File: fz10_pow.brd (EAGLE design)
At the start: 107 x 100 mm, 85 parts

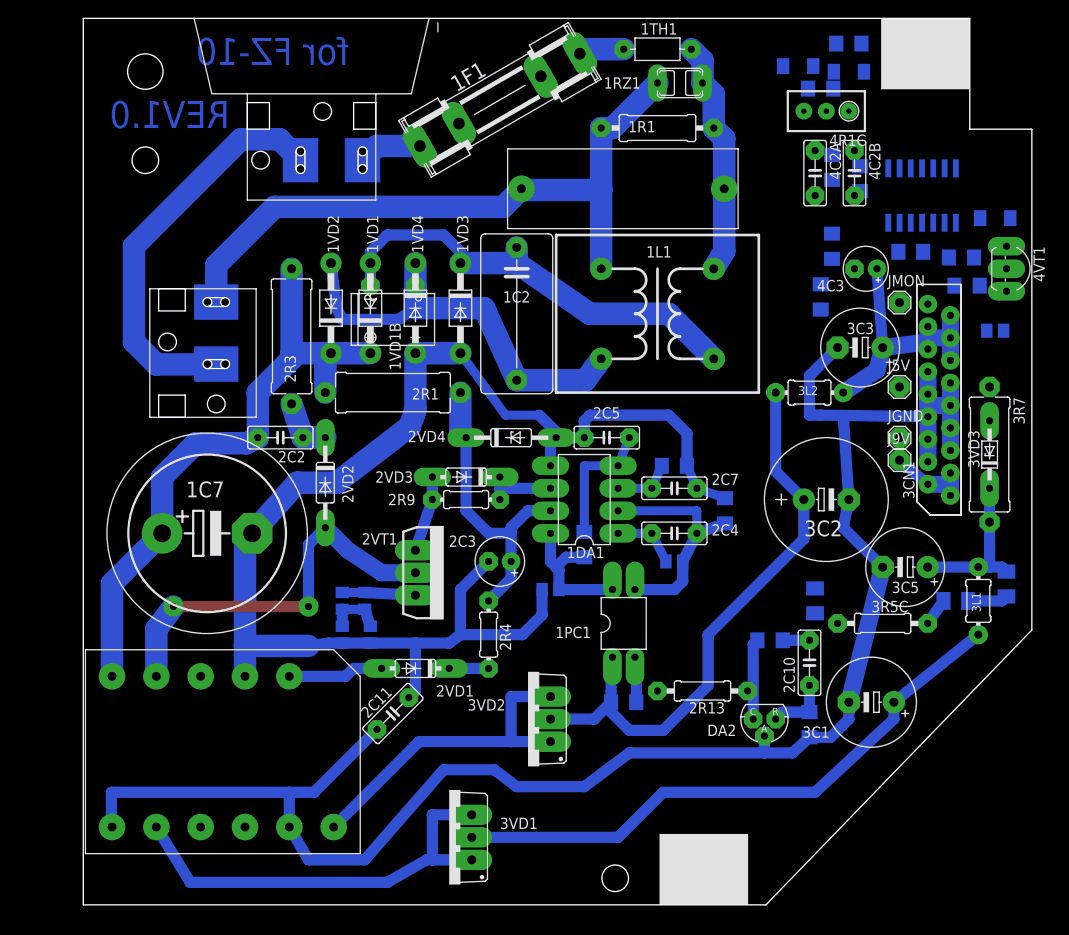
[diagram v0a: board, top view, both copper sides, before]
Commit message: .
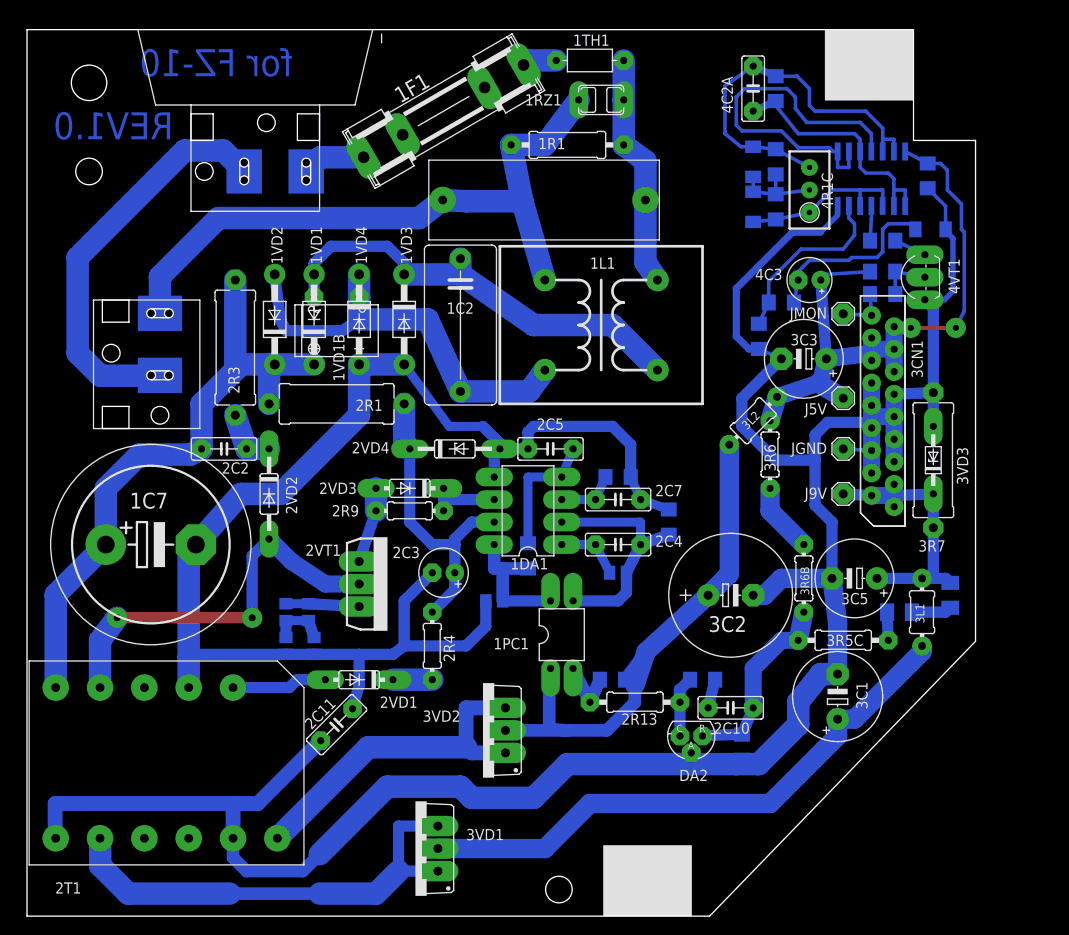
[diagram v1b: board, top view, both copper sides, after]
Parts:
- removed 4C2B: (no value), rcl:C050-025X075
- removed 4C2D: (no value), rcl:C1206
- added 3R6B: 0, rcl:0204/7
- 3R6: device rcl:M1206 -> rcl:0204/7
- 4R6: device rcl:M0805 -> rcl:R1206
- moved 4R1B 20.2 mm to (84.5, 80.0), turned to 270 degrees
- moved 4VD2 18.7 mm to (81.9, 80.0), turned to 270 degrees
- moved 3R6 17.3 mm to (83.8, 52.1), flipped to the top
- moved 3C2 15.3 mm to (79.4, 36.2)
- moved 4C2C 13.9 mm to (84.5, 93.3), turned to 90 degrees
- moved 4R6 13.4 mm to (96.5, 70.2)
- moved 4VD1 11.9 mm to (81.9, 85.1), turned to 90 degrees
- moved 4C2A 11.8 mm to (81.9, 93.3), turned to 90 degrees
- moved 4R4 10.8 mm to (96.5, 76.2)
- moved 1R1 10.3 mm to (61.0, 87.0)
- moved 2C10 10.2 mm to (79.4, 23.5), turned to 180 degrees
- moved 4R1A 9.69 mm to (84.5, 85.1), turned to 270 degrees
- moved 4VT1 9.26 mm to (101.3, 72.1), turned to 90 degrees
- moved 1RZ1 9.09 mm to (64.8, 92.1)
- moved 4R1C 9.09 mm to (88.3, 81.9), turned to 0 degrees
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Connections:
- new net N$43: 3R6.1, 3R6B.2
- net N$1: now also 4DD1.12, 4DD1.13; no longer 4C2B.2, 4C2D.2, 4DD1.1, 4DD1.2
- net N$19: now also 4DD1.1, 4DD1.10, 4DD1.2; no longer 4C2B.1, 4C2D.1, 4DD1.12, 4DD1.13, 4DD1.4
- net N$2: now also 4DD1.11, 4DD1.8, 4DD1.9; no longer 4DD1.3, 4DD1.5, 4DD1.6
- net N$25: now also 4DD1.4; no longer 4DD1.10
- net N$31: now also 4DD1.6; no longer 4DD1.8
- net N$42: now also 3R6B.1; no longer 3R6.1
- net N$7: now also 4DD1.3, 4DD1.5; no longer 4DD1.11, 4DD1.9
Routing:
- net GND: track 196.5 -> 277.0 mm
- net +5V: track 31.4 -> 75.2 mm, vias 0 -> 2
- net N$1: track 0.00 -> 43.5 mm
- net N$2: track 0.00 -> 41.4 mm
- net N$19: track 0.00 -> 28.3 mm
- net N$35: track 0.00 -> 20.7 mm
- net N$31: track 0.00 -> 20.5 mm
- net N$7: track 0.00 -> 19.4 mm
- net N$42: track 7.16 -> 21.8 mm
- net N$10: track 0.00 -> 10.3 mm
- net N$43: track 0.00 -> 7.93 mm
- net N$29: track 0.00 -> 5.94 mm
- net MON: track 0.00 -> 5.61 mm
- net N$13: track 66.4 -> 62.3 mm
- net N$25: track 0.00 -> 3.92 mm
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
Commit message: .
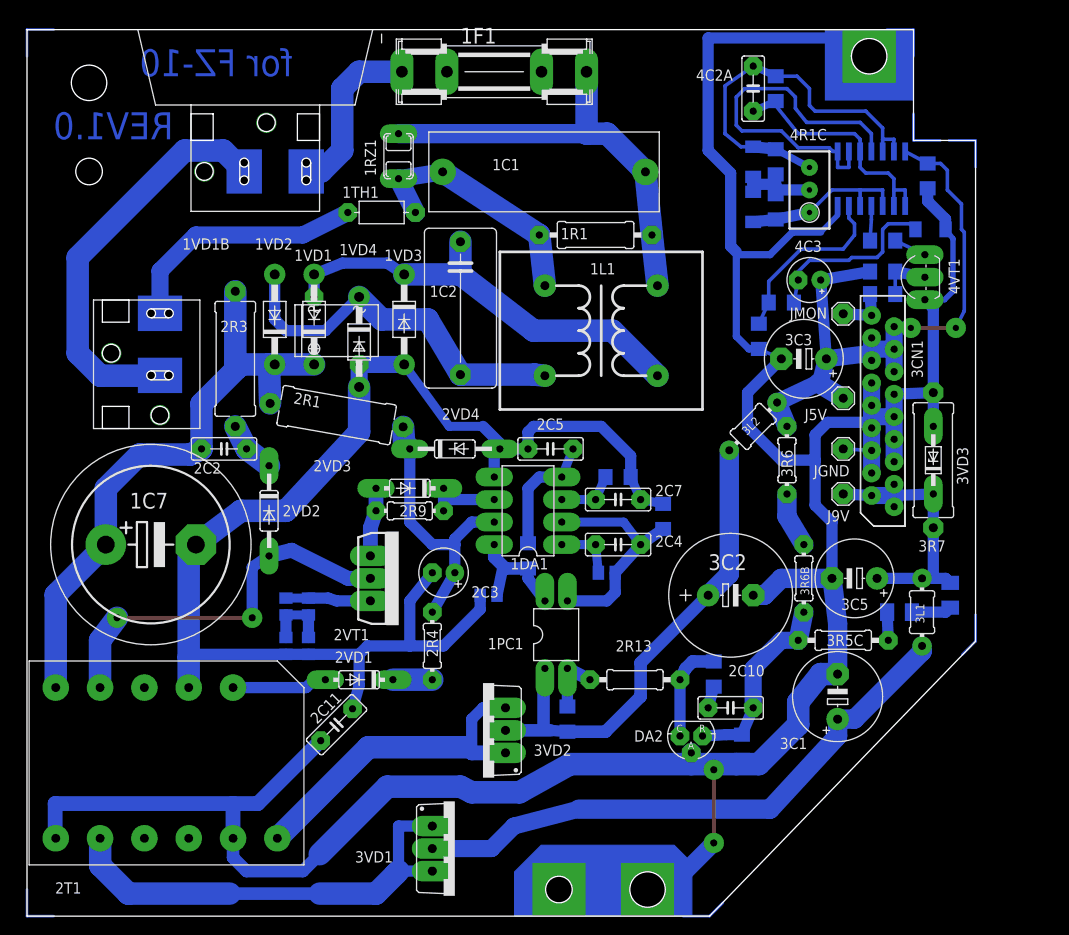
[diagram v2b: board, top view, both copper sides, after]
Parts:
- 2R8: value 68k *80ruw -> 68k *80khz
- 2VD4: value (none) -> 22v
- 4C1: value (none) -> 100n
- moved 1TH1 29.1 mm to (40.0, 79.4)
- moved 1RZ1 23.7 mm to (41.9, 85.7), turned to 270 degrees
- moved 1R1 10.6 mm to (64.1, 76.8)
- moved 1F1 7.24 mm to (52.7, 95.2), turned to 0 degrees
- moved 2R12 6.75 mm to (61.0, 22.2), turned to 270 degrees
- moved 3VD1 4.45 mm to (48.3, 7.62), turned to 270 degrees
- moved 1C1 3.17 mm to (60.3, 84.5)
- moved 1VD4 2.54 mm to (37.5, 64.8)
- moved 2R13 2.54 mm to (68.6, 26.7)
- moved 3R6 2.01 mm to (85.7, 51.4)
- moved 1C2 1.91 mm to (48.9, 68.6)
- moved 2VD2 1.91 mm to (27.3, 45.7)
- moved 2R14 1.42 mm to (77.5, 27.3), turned to 270 degrees
- moved 2VT1 1.42 mm to (38.7, 38.1)
- moved 2R3 1.27 mm to (23.5, 62.9)
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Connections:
- net N$9 renamed +16IN
- removed net N$36: 1F1.2A, 1TH1.1
- new net N$9: 1TH1.1, PCB.SW1
- net N$32: now also 1TH1.2; no longer PCB.SW1
- net N$33: now also 1F1.2A; no longer 1TH1.2
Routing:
- net GND: track 277.0 -> 330.3 mm, vias 0 -> 2
- net N$32: track 74.3 -> 28.1 mm
- net N$9: track 0.00 -> 28.3 mm
- net N$33: track 26.4 -> 49.5 mm
- net N$18: track 7.13 -> 19.5 mm
- net N$13: track 62.3 -> 56.6 mm
- net N$44: track 47.7 -> 42.3 mm
- net N$14: track 6.81 -> 11.3 mm
- net N$36: track 3.89 -> 0.00 mm
- net +16IN: track 34.3 -> 31.3 mm
- net -IN: track 152.3 -> 150.1 mm
- net N$20: track 15.6 -> 13.5 mm
- net N$43: track 7.93 -> 6.24 mm
- net N$40: track 27.0 -> 25.5 mm
- net N$17: track 45.4 -> 44.0 mm
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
